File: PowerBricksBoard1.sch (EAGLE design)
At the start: 16 parts

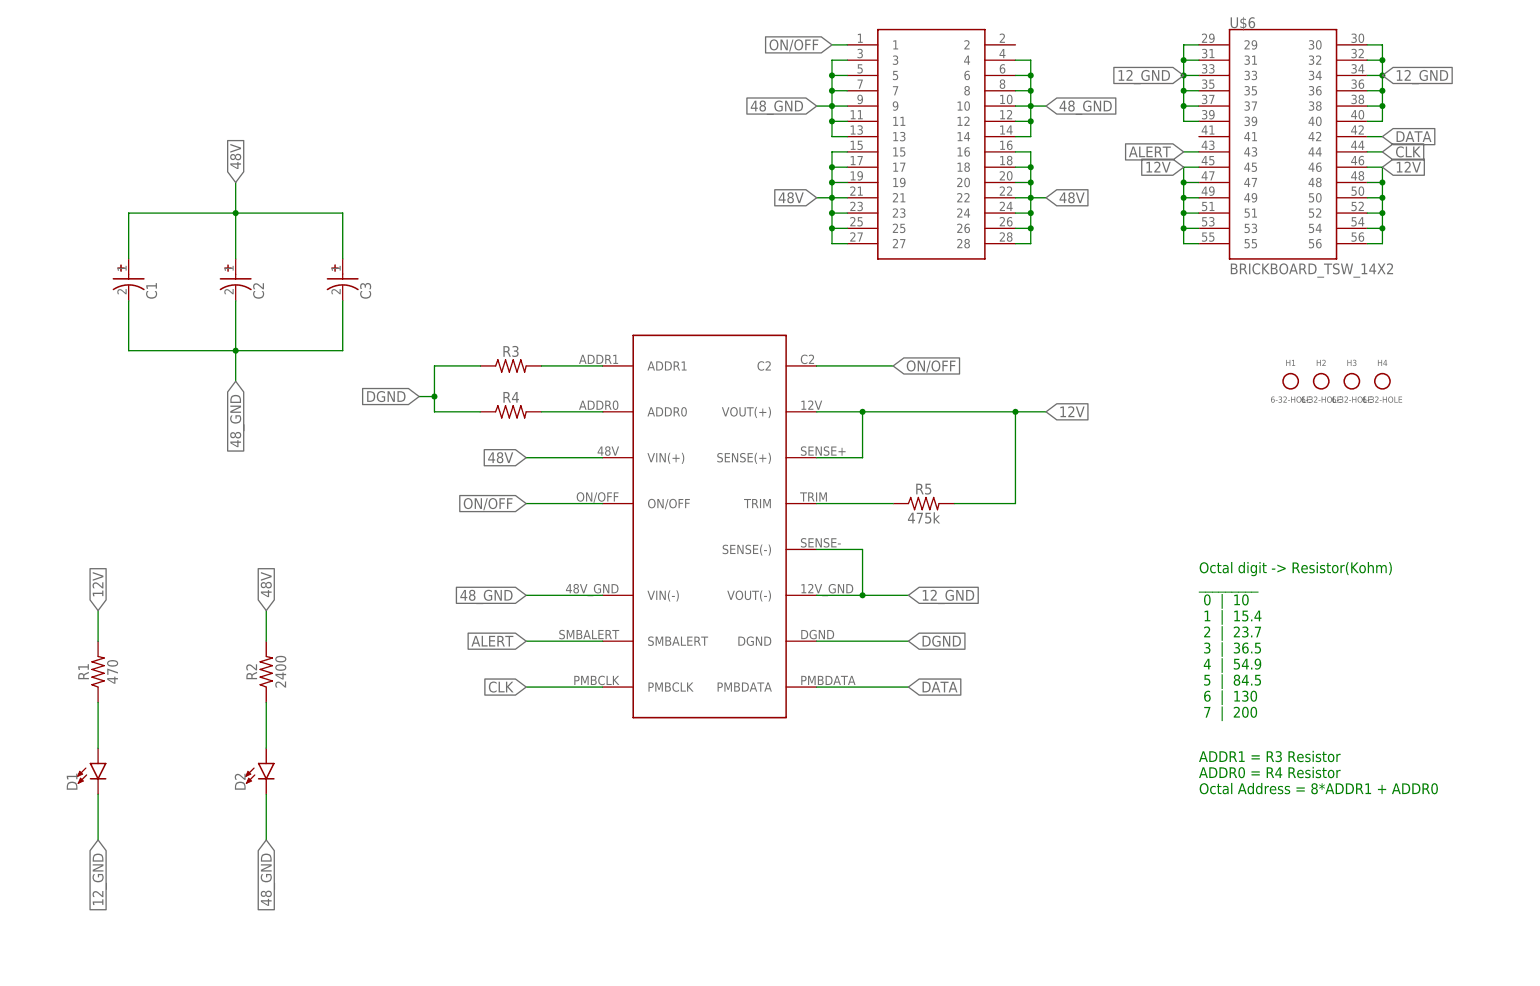
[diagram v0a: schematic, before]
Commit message: test
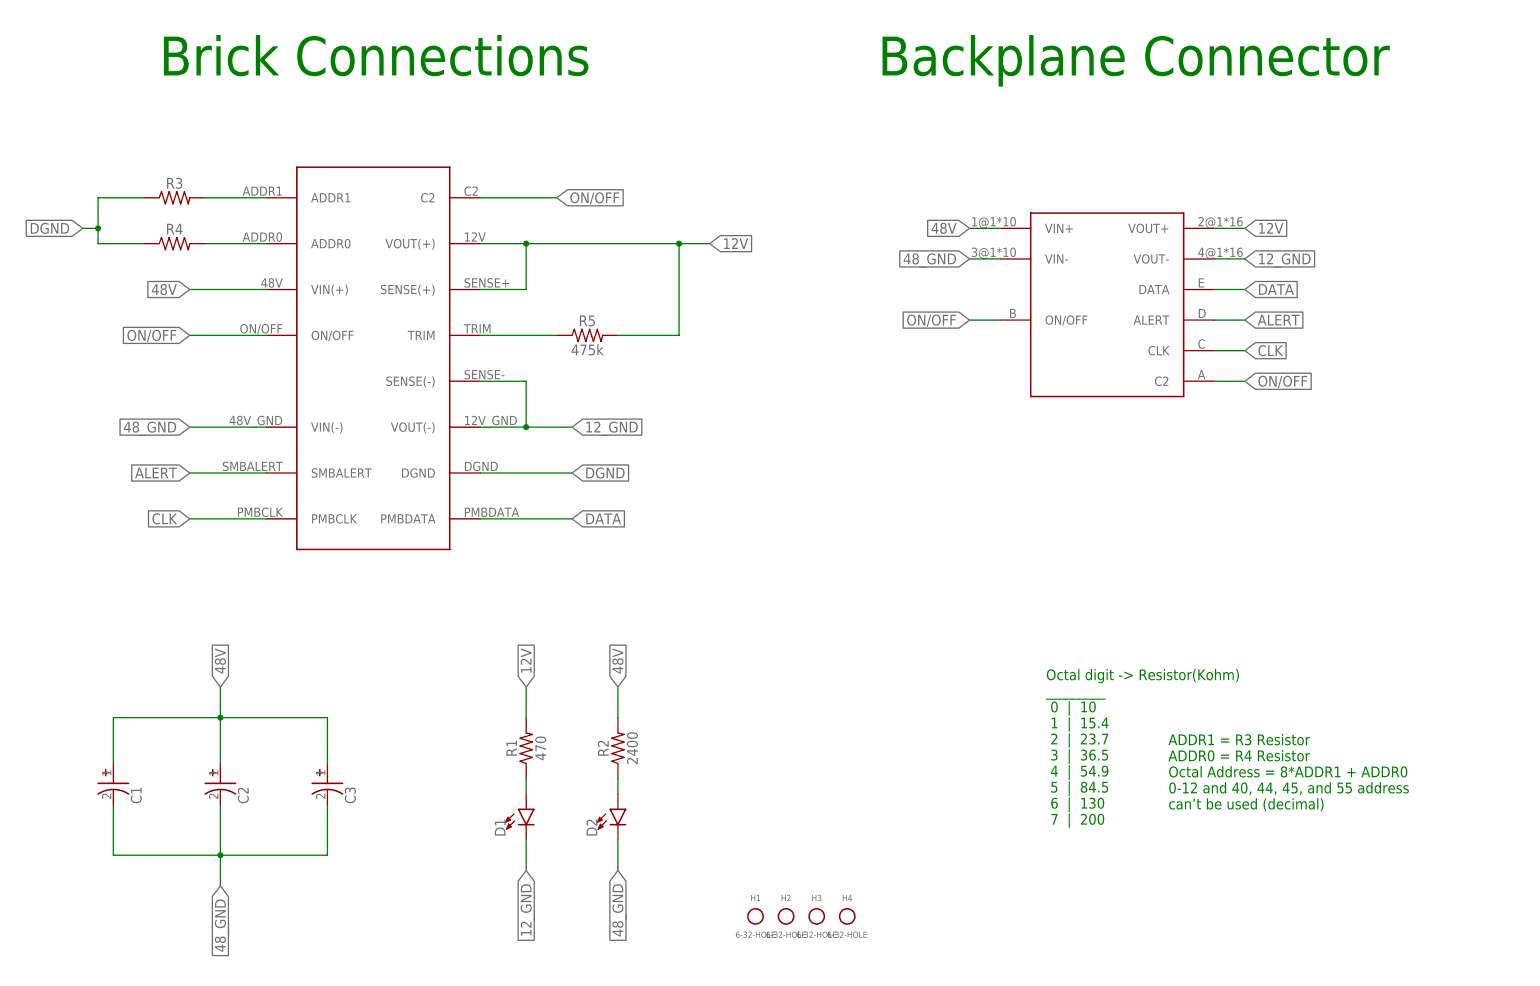
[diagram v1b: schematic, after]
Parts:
- removed U$6: BRICKBOARD_TSW_14X2, Dist_to_Brickboard_Connector_brick:BRICKBOARD_TSW_14X2
- added U$2: BRICK2DIST, Brick_Dist_Connector:BRICK2DIST
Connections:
- net 12V: now also U$2.VOUT+; no longer U$6.45, U$6.46, U$6.47, U$6.48, U$6.49, U$6.50, U$6.51, U$6.52, U$6.53, U$6.54, U$6.55, U$6.56
- net 12_GND: now also U$2.VOUT-; no longer U$6.29, U$6.30, U$6.31, U$6.32, U$6.33, U$6.34, U$6.35, U$6.36, U$6.37, U$6.38, U$6.39, U$6.40
- net 48V: now also U$2.VIN+; no longer U$6.15, U$6.16, U$6.17, U$6.18, U$6.19, U$6.20, U$6.21, U$6.22, U$6.23, U$6.24, U$6.25, U$6.26, U$6.27, U$6.28
- net 48_GND: now also U$2.VIN-; no longer U$6.10, U$6.11, U$6.12, U$6.13, U$6.14, U$6.3, U$6.4, U$6.5, U$6.6, U$6.7, U$6.8, U$6.9
- net ALERT: now also U$2.ALERT; no longer U$6.43
- net CLK: now also U$2.CLK; no longer U$6.44
- net DATA: now also U$2.DATA; no longer U$6.42
- net ON/OFF: now also U$2.C2, U$2.ON/OFF; no longer U$6.1
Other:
- note added: "ADDR1 = R3 Resistor ADDR0 = R4 Resistor Octal Address = 8*ADDR1 + ADDR0 0-12 and 40, 44, 45, and 55 address can’t be used (decimal)"
- note added: "Backplane Connector"
- note added: "Brick Connections"
- note removed: "ADDR1 = R3 Resistor ADDR0 = R4 Resistor Octal Address = 8*ADDR1 + ADDR0"
- moved on the sheet: C1, C2, C3, D1, D2, H1, H2, H3, H4, R1, R2, R3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
